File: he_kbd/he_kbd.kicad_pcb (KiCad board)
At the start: 2 copper layers, 162.2 x 126.5 mm, 270 parts, among them J1 AudioJack4, J2 Conn_01x08_Pin, J3 AudioJack4, J4 Conn_01x08_Pin

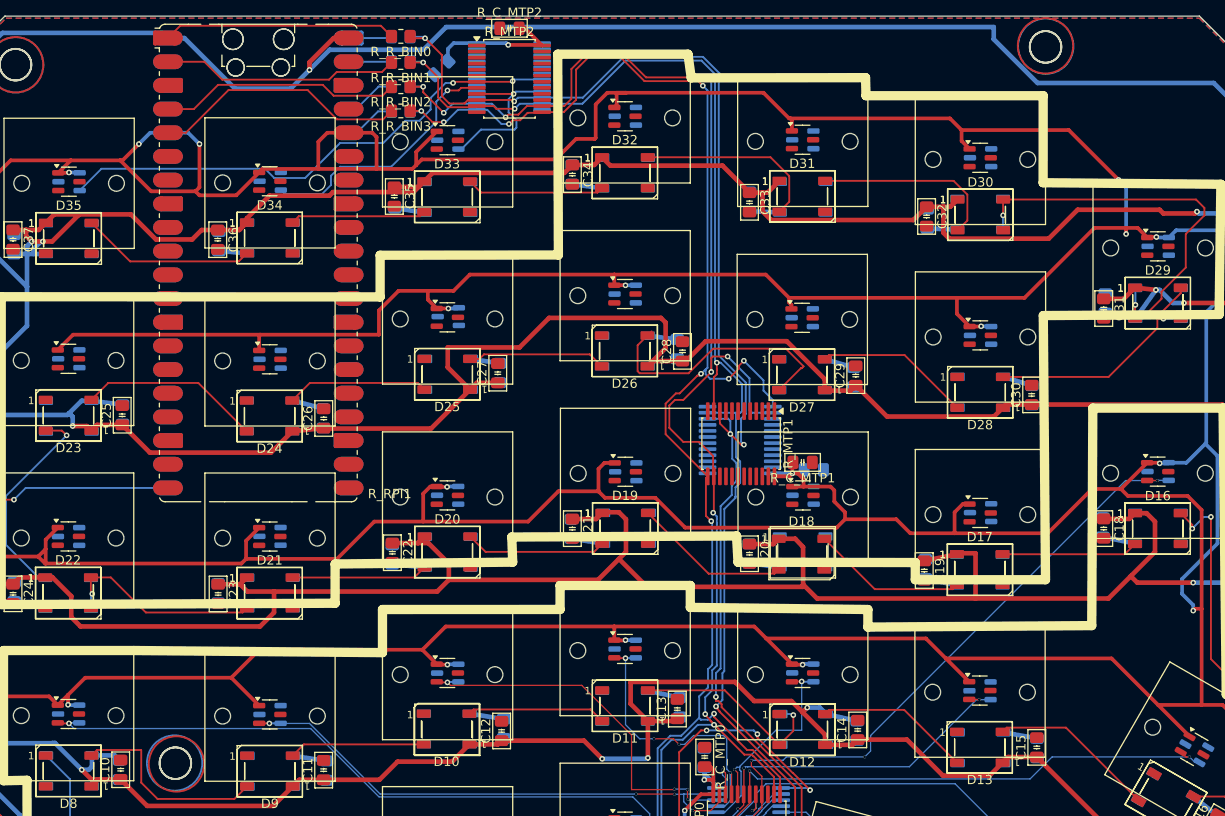
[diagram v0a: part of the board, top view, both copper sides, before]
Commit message: mtp1 almost finished!!
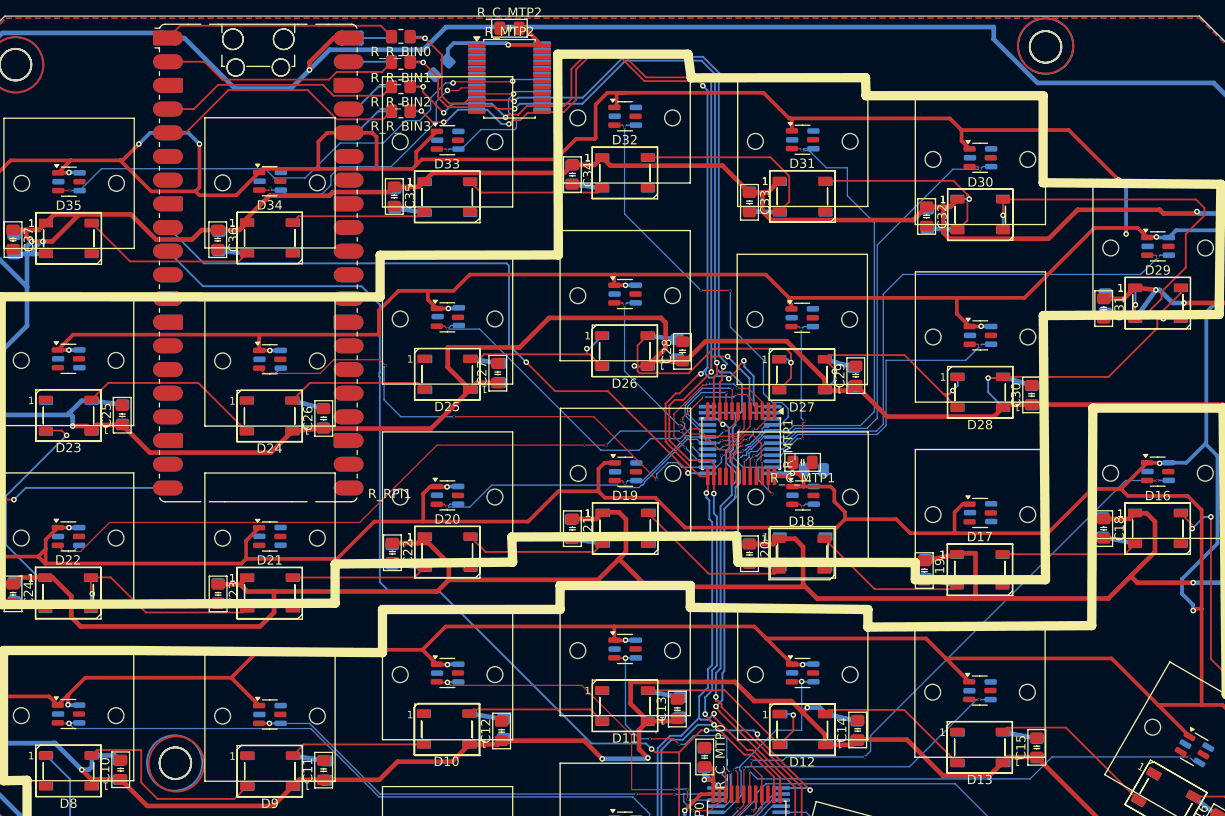
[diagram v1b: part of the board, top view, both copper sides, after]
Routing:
- net /ADC_0: track 34.1 -> 128.7 mm, vias 3 -> 4
- net /hesig22: track 0.00 -> 90.0 mm, vias 0 -> 8
- net /ADC_1: track 0.00 -> 73.9 mm, vias 0 -> 2
- net /hesig24: track 0.00 -> 69.5 mm, vias 0 -> 7
- net /hesig29: track 0.00 -> 66.1 mm, vias 0 -> 2
- net /hesig25: track 0.00 -> 54.9 mm, vias 0 -> 4
- net /hesig31: track 0.00 -> 54.8 mm, vias 0 -> 2
- net /hesig30: track 0.00 -> 54.4 mm, vias 0 -> 2
- net /hesig32: track 0.00 -> 53.8 mm, vias 0 -> 4
- net /hesig20: track 0.00 -> 40.5 mm, vias 0 -> 2
- net /hesig28: track 0.00 -> 38.1 mm, vias 0 -> 2
- net /hesig26: track 0.00 -> 33.6 mm, vias 0 -> 3
- net /hesig27: track 0.00 -> 22.2 mm, vias 0 -> 4
- net /hesig23: track 0.00 -> 19.8 mm, vias 0 -> 3
- net /hesig19: track 0.00 -> 17.3 mm, vias 0 -> 2
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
